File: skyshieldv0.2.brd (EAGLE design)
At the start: 17.8 x 43.2 mm, 21 parts, among them IC2 MCP1702-5, J1 HEAD15-NOSS, J2 HEAD15-NOSS-1

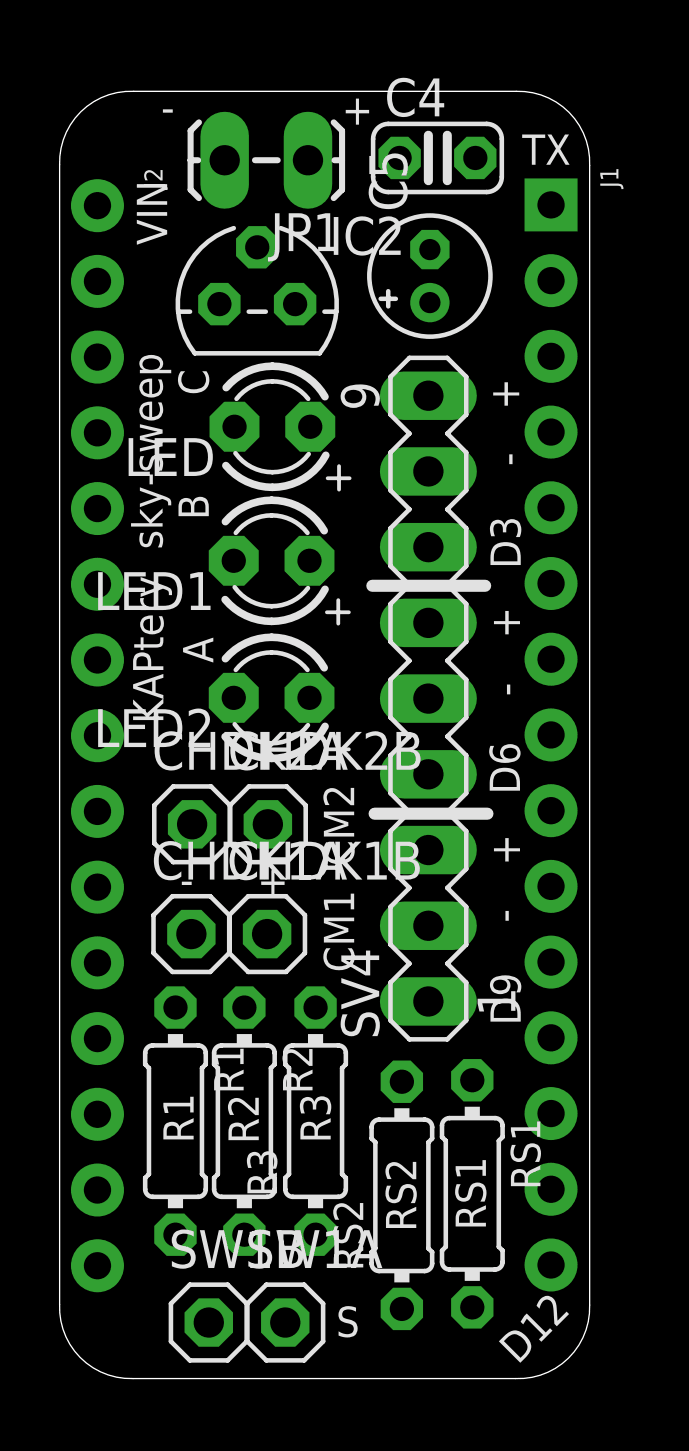
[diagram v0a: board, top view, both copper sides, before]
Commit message: update
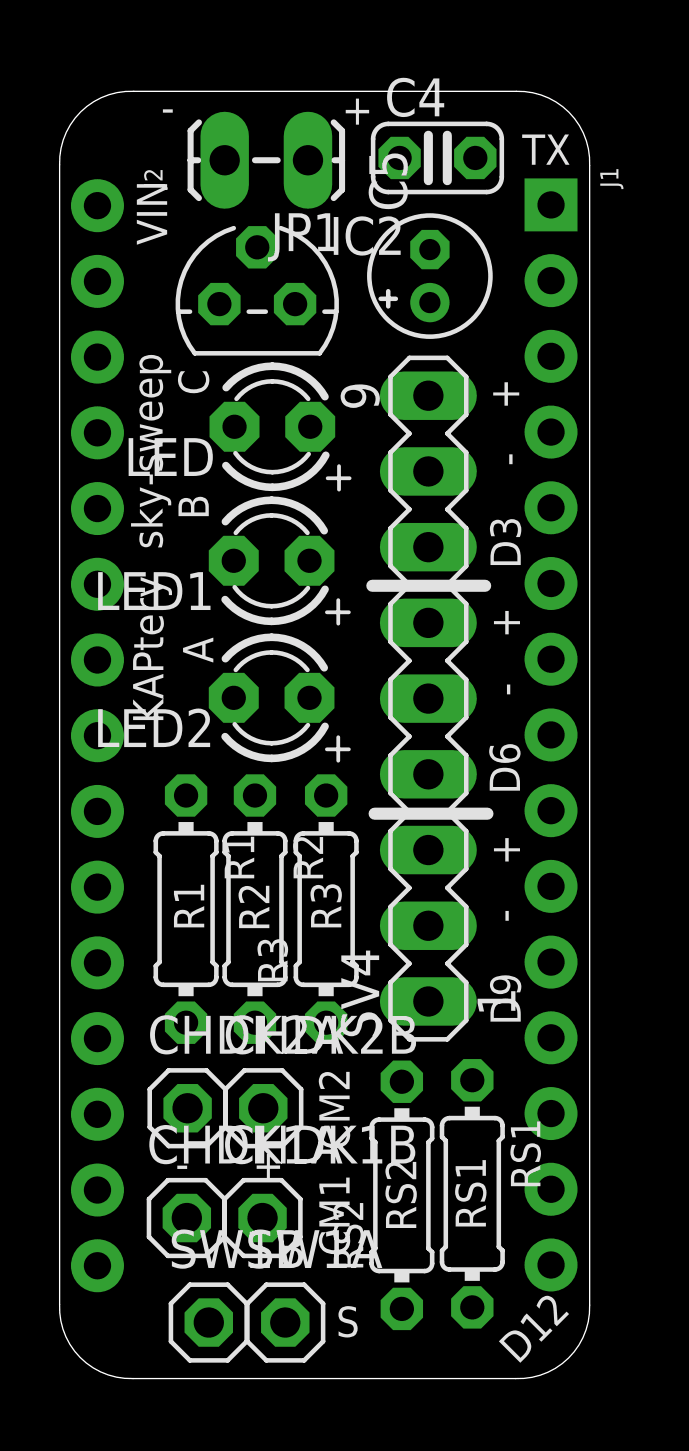
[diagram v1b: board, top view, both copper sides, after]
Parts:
- moved CHDK1A 9.53 mm to (4.27, 5.38)
- moved CHDK1B 9.53 mm to (6.81, 5.38)
- moved CHDK2A 9.53 mm to (4.29, 9.07)
- moved CHDK2B 9.53 mm to (6.83, 9.07)
- moved R1 7.12 mm to (4.24, 15.7)
- moved R2 7.12 mm to (6.55, 15.7)
- moved R3 7.12 mm to (8.94, 15.7)
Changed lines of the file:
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@@
 <wire x1="10.4902" y1="26.5938" x2="14.2748" y2="26.5938" width="0.4064" layer="21"/>
 <wire x1="10.5664" y1="18.9484" x2="14.351" y2="18.9484" width="0.4064" layer="21"/>
-<text x="4.0386" y="16.2306" size="1.016" layer="21" ratio="15">-</text>
-<text x="6.6294" y="16.1798" size="1.016" layer="21" ratio="15">+</text>
-<text x="8.8646" y="16.383" size="1.016" layer="21" ratio="15" rot="R270">CM1</text>
-<text x="8.8646" y="19.939" size="1.016" layer="21" ratio="15" rot="R270">CM2</text>
+<text x="3.8862" y="6.7056" size="1.016" layer="21" ratio="15">-</text>
+<text x="6.477" y="6.6548" size="1.016" layer="21" ratio="15">+</text>
+<text x="8.7122" y="6.858" size="1.016" layer="21" ratio="15" rot="R270">CM1</text>
+<text x="8.7122" y="10.414" size="1.016" layer="21" ratio="15" rot="R270">CM2</text>
 <text x="9.271" y="1.397" size="1.016" layer="21" ratio="15">S</text>
-<text x="4.4958" y="7.8994" size="1.016" layer="21" ratio="15" rot="R90">R1</text>
-<text x="6.6802" y="7.874" size="1.016" layer="21" ratio="15" rot="R90">R2</text>
-<text x="9.0932" y="7.8994" size="1.016" layer="21" ratio="15" rot="R90">R3</text>
+<text x="4.8514" y="15.0114" size="1.016" layer="21" ratio="15" rot="R90">R1</text>
+<text x="7.0358" y="14.986" size="1.016" layer="21" ratio="15" rot="R90">R2</text>
+<text x="9.4488" y="15.0114" size="1.016" layer="21" ratio="15" rot="R90">R3</text>
 <text x="14.3002" y="4.9784" size="1.016" layer="21" ratio="15" rot="R90">RS1</text>
 <text x="11.9634" y="4.9276" size="1.016" layer="21" ratio="15" rot="R90">RS2</text>
@@
 <element name="J1" library="MyCON2" package="HEAD15-NOSS" value="HEAD15-NOSS" x="16.4846" y="39.37" rot="R270"/>
 <element name="J2" library="MyCON2" package="HEAD15-NOSS-1" value="HEAD15-NOSS-1" x="1.27" y="39.3446" rot="R270"/>
-<element name="R1" library="rcl" package="0204/7" value="10K" x="3.8862" y="8.636" rot="R270"/>
+<element name="R1" library="rcl" package="0204/7" value="10K" x="4.2418" y="15.748" rot="R270"/>
 <element name="IC2" library="JeeLabs" package="TO92" value="MCP1702-5" x="6.6294" y="36.0426"/>
 <element name="C5" library="resistor" package="E1,8-4" value="10µ" x="12.4206" y="36.9824" rot="R90"/>
@@
 <attribute name="VALUE" x="15.2908" y="22.8092" size="1.27" layer="27" ratio="10" rot="R90"/>
 </element>
-<element name="R2" library="rcl" package="0204/7" value="10K" x="6.1976" y="8.636" rot="R270"/>
+<element name="R2" library="rcl" package="0204/7" value="10K" x="6.5532" y="15.748" rot="R270"/>
 <element name="LED1" library="adafruit" package="LED3MM" value="POWERLED" x="7.112" y="27.432" rot="R180"/>
-<element name="R3" library="rcl" package="0204/7" value="10K" x="8.5852" y="8.636" rot="R90"/>
+<element name="R3" library="rcl" package="0204/7" value="10K" x="8.9408" y="15.748" rot="R90"/>
 <element name="LED2" library="adafruit" package="LED3MM" value="POWERLED" x="7.112" y="22.8346" rot="R180"/>
 <element name="RS2" library="rcl" package="0204/7" value="10K" x="11.4808" y="6.1468" rot="R90"/>
 <element name="RS1" library="rcl" package="0204/7" value="100" x="13.843" y="6.1976" rot="R270"/>
-<element name="CHDK1A" library="pinhead" package="1X01" value="" x="4.4196" y="14.9098"/>
-<element name="CHDK1B" library="pinhead" package="1X01" value="" x="6.9596" y="14.9098"/>
-<element name="CHDK2A" library="pinhead" package="1X01" value="" x="4.445" y="18.5928"/>
-<element name="CHDK2B" library="pinhead" package="1X01" value="" x="6.985" y="18.5928"/>
+<element name="CHDK1A" library="pinhead" package="1X01" value="" x="4.2672" y="5.3848"/>
+<element name="CHDK1B" library="pinhead" package="1X01" value="" x="6.8072" y="5.3848"/>
+<element name="CHDK2A" library="pinhead" package="1X01" value="" x="4.2926" y="9.0678"/>
+<element name="CHDK2B" library="pinhead" package="1X01" value="" x="6.8326" y="9.0678"/>
 <element name="SW1B" library="pinhead" package="1X01" value="" x="5.0038" y="1.8796"/>
 <element name="SW1A" library="pinhead" package="1X01" value="" x="7.5692" y="1.8796"/>
@@
 <contactref element="J2" pad="9"/>
 <contactref element="R2" pad="1"/>
-<wire x1="6.1976" y1="12.446" x2="1.27" y2="19.0246" width="0" layer="19" extent="1-1"/>
+<wire x1="6.5532" y1="19.558" x2="1.27" y2="19.0246" width="0" layer="19" extent="1-1"/>
 </signal>
 <signal name="A4">
 <contactref element="J2" pad="8"/>
 <contactref element="R3" pad="1"/>
-<wire x1="8.5852" y1="4.826" x2="1.27" y2="21.5646" width="0" layer="19" extent="1-1"/>
+<wire x1="8.9408" y1="11.938" x2="1.27" y2="21.5646" width="0" layer="19" extent="1-1"/>
 </signal>
 <signal name="A5">
@@
 <wire x1="5.842" y1="27.432" x2="5.8674" y2="31.9278" width="0" layer="19" extent="1-1"/>
 <wire x1="5.842" y1="22.8346" x2="5.842" y2="27.432" width="0" layer="19" extent="1-1"/>
-<wire x1="6.9596" y1="14.9098" x2="5.842" y2="22.8346" width="0" layer="19" extent="1-1"/>
-<wire x1="6.985" y1="18.5928" x2="6.9596" y2="14.9098" width="0" layer="19" extent="1-1"/>
+<wire x1="6.8072" y1="5.3848" x2="5.842" y2="22.8346" width="0" layer="19" extent="1-1"/>
+<wire x1="6.8326" y1="9.0678" x2="6.8072" y2="5.3848" width="0" layer="19" extent="1-1"/>
 <wire x1="5.5372" y1="40.8686" x2="5.3594" y2="36.0426" width="0" layer="19" extent="1-1"/>
-<wire x1="12.3698" y1="17.7292" x2="6.9596" y2="14.9098" width="0" layer="19" extent="1-1"/>
+<wire x1="12.3698" y1="17.7292" x2="6.8072" y2="5.3848" width="0" layer="19" extent="1-1"/>
 <wire x1="12.3698" y1="25.3492" x2="5.842" y2="27.432" width="0" layer="19" extent="1-1"/>
-<wire x1="5.0038" y1="1.8796" x2="6.985" y2="18.5928" width="0" layer="19" extent="1-1"/>
+<wire x1="5.0038" y1="1.8796" x2="6.8326" y2="9.0678" width="0" layer="19" extent="1-1"/>
 </signal>
 <signal name="VCC" class="1">
@@
 <contactref element="R3" pad="2"/>
 <contactref element="LED2" pad="A"/>
-<wire x1="8.5852" y1="12.446" x2="8.382" y2="22.8346" width="0" layer="19" extent="1-1"/>
+<wire x1="8.9408" y1="19.558" x2="8.382" y2="22.8346" width="0" layer="19" extent="1-1"/>
 </signal>
 <signal name="N$2">
 <contactref element="R2" pad="2"/>
 <contactref element="LED1" pad="A"/>
-<wire x1="6.1976" y1="4.826" x2="8.382" y2="27.432" width="0" layer="19" extent="1-1"/>
+<wire x1="6.5532" y1="11.938" x2="8.382" y2="27.432" width="0" layer="19" extent="1-1"/>
 </signal>
 <signal name="N$3">
 <contactref element="R1" pad="2"/>
 <contactref element="LED" pad="A"/>
-<wire x1="3.8862" y1="4.826" x2="8.4074" y2="31.9278" width="0" layer="19" extent="1-1"/>
+<wire x1="4.2418" y1="11.938" x2="8.4074" y2="31.9278" width="0" layer="19" extent="1-1"/>
 </signal>
 <signal name="N$4">
@@
 <contactref element="J2" pad="10"/>
 <contactref element="R1" pad="1"/>
-<wire x1="3.8862" y1="12.446" x2="1.27" y2="16.4846" width="0" layer="19" extent="1-1"/>
+<wire x1="4.2418" y1="19.558" x2="1.27" y2="16.4846" width="0" layer="19" extent="1-1"/>
 </signal>
 <signal name="A1">
 <contactref element="J2" pad="11"/>
 <contactref element="CHDK2A" pad="1"/>
-<wire x1="1.27" y1="13.9446" x2="4.445" y2="18.5928" width="0" layer="19" extent="1-1"/>
+<wire x1="1.27" y1="13.9446" x2="4.2926" y2="9.0678" width="0" layer="19" extent="1-1"/>
 </signal>
 <signal name="A0">
 <contactref element="J2" pad="12"/>
 <contactref element="CHDK1A" pad="1"/>
-<wire x1="1.27" y1="11.4046" x2="4.4196" y2="14.9098" width="0" layer="19" extent="1-1"/>
+<wire x1="1.27" y1="11.4046" x2="4.2672" y2="5.3848" width="0" layer="19" extent="1-1"/>
 </signal>
 <signal name="N$5">
